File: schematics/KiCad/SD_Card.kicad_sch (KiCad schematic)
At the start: 13 parts, among them J6 Micro_SD_Card_Det_Hirose_DM3AT, U14 LP2950-3.3, U16 74HC4050

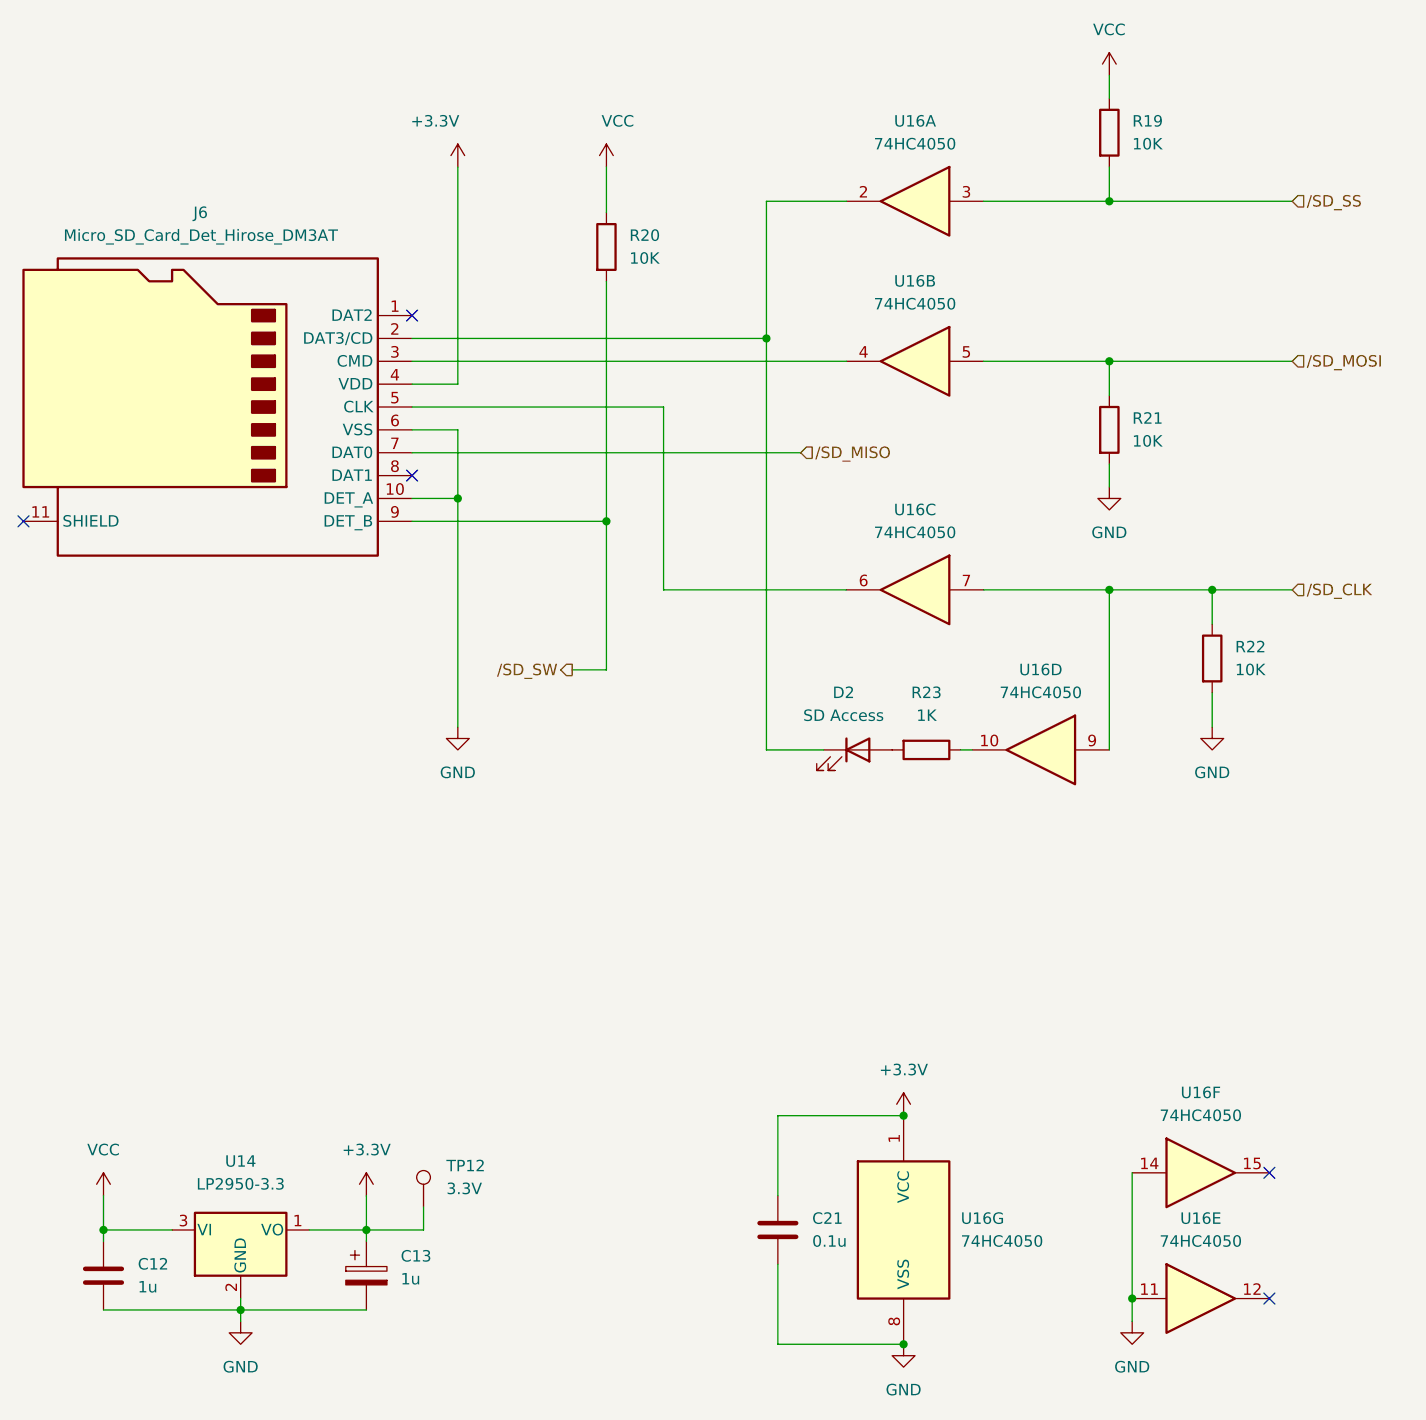
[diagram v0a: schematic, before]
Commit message: Update schematics
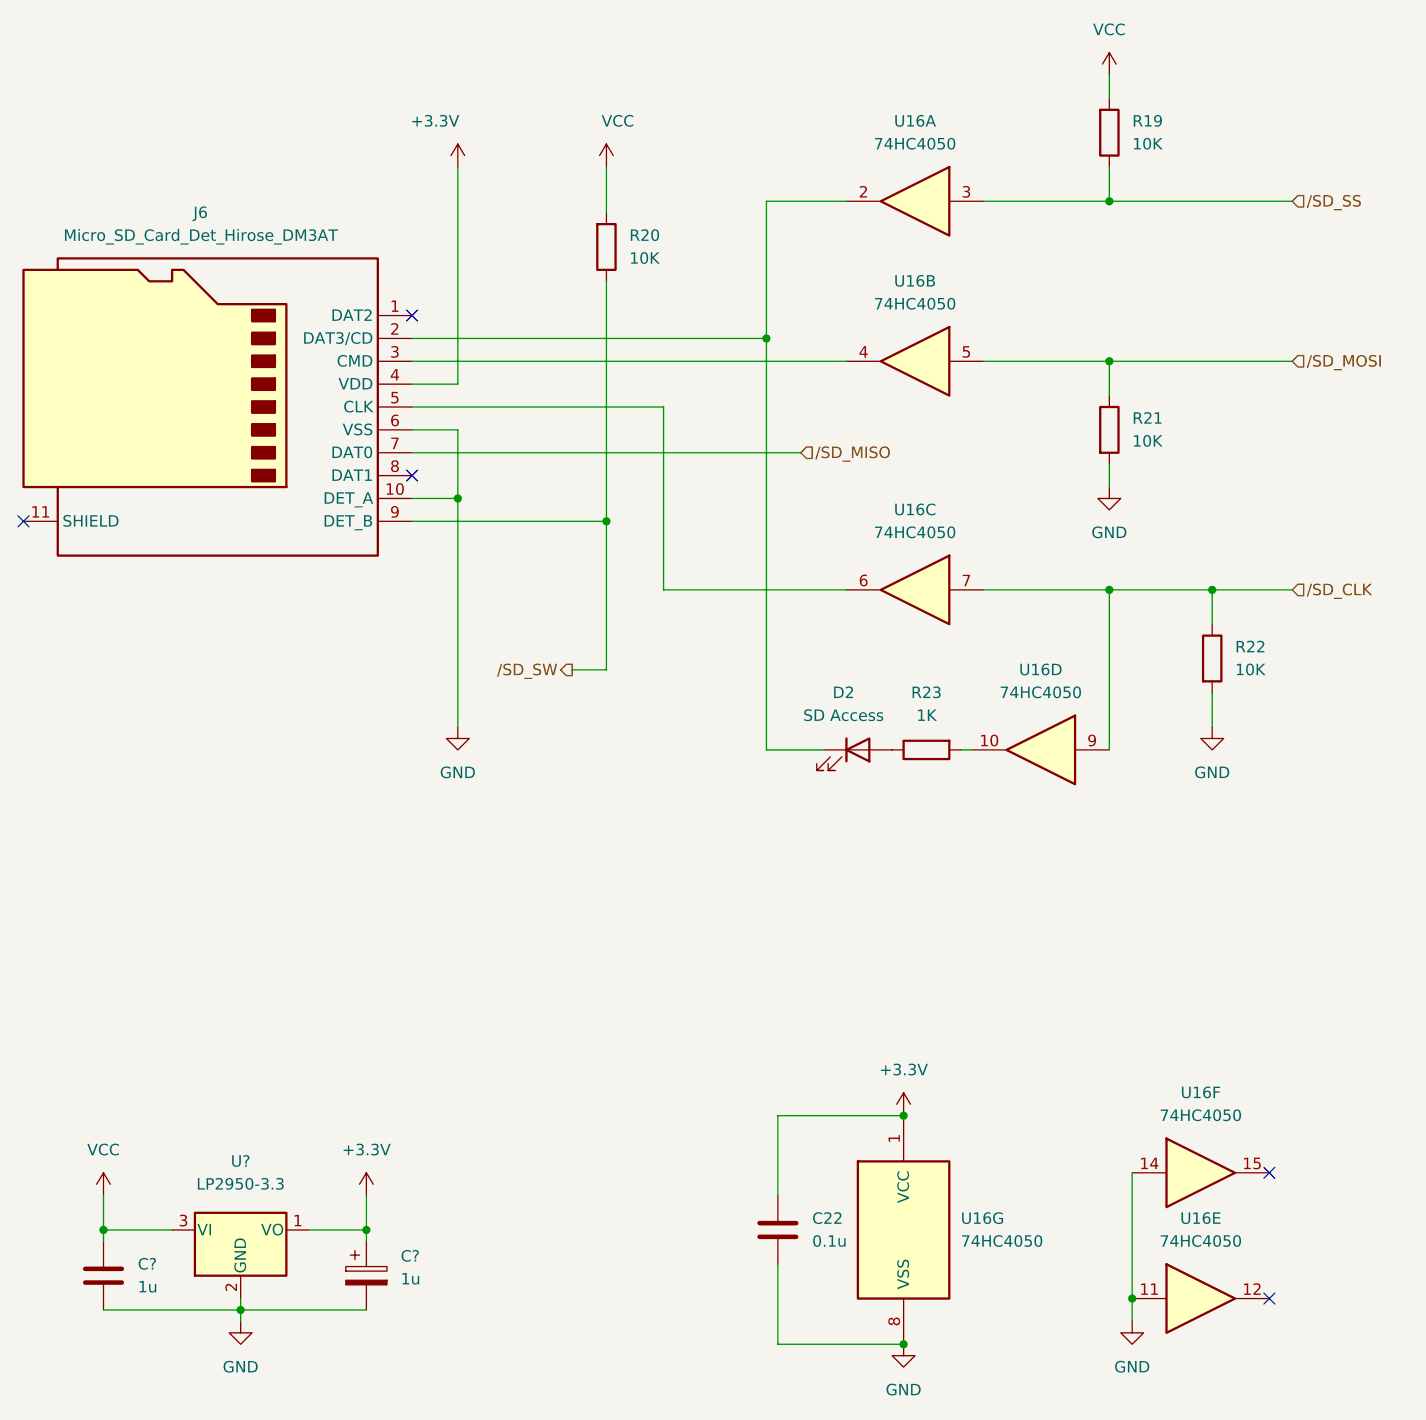
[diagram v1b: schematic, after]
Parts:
- removed TP12: 3.3V, TestPoint:TestPoint_Loop_D2.50mm_Drill1.0mm, symbol Connector:TestPoint
- C?: renamed from C12; footprint Capacitor_THT:CP_Radial_Tantal_D5.0mm_P2.50mm -> Capacitor_THT:C_Disc_D3.8mm_W2.6mm_P2.50mm
- C?: renamed from C13; footprint Capacitor_THT:CP_Radial_Tantal_D5.0mm_P2.50mm -> Capacitor_THT:CP_Radial_D5.0mm_P2.50mm
- renumbered C21 to C22, U14 to U?
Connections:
- net VCC: now also R19.2, R20.2; no longer R19.1, R20.1
- net /SD_SS: now also R19.1; no longer R19.2
- net /SD_SW: now also R20.1; no longer R20.2
- net at D2.2 (A): now also R23.1; no longer R23.2
- net at U16.10: now also R23.2; no longer R23.1
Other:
- moved on the sheet: R23

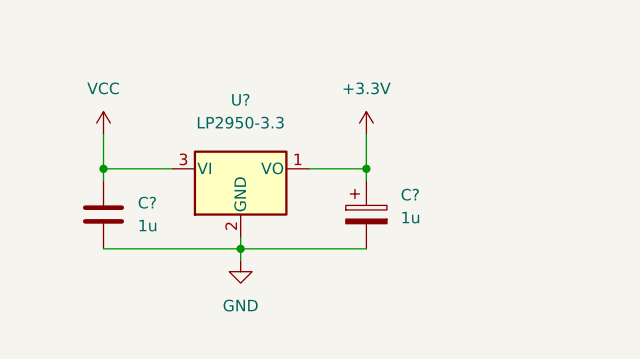
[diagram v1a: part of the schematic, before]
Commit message: Update for PCB design
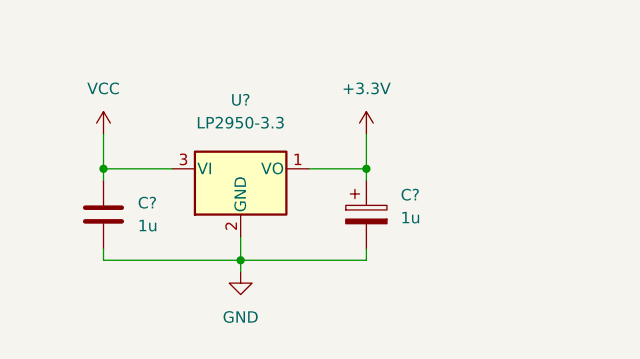
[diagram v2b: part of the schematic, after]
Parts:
- U?: footprint Package_TO_SOT_THT:TO-92_Inline -> Package_TO_SOT_THT:TO-92_Inline_Wide
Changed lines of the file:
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@@
     (company "By 46nori")
   )
-  (junction (at 49.53 167.64) (diameter 0) (color 0 0 0 0)
+  (junction (at 49.53 168.91) (diameter 0) (color 0 0 0 0)
   )
   (junction (at 107.95 59.69) (diameter 0) (color 0 0 0 0)
@@
     (stroke (width 0) (type default))
   )
+  (wire (pts (xy 63.5 168.91) (xy 63.5 167.64))
+    (stroke (width 0) (type default))
+  )
   (wire (pts (xy 109.22 162.56) (xy 109.22 171.45))
     (stroke (width 0) (type default))
@@
     (stroke (width 0) (type default))
   )
-  (wire (pts (xy 49.53 166.37) (xy 49.53 167.64))
-    (stroke (width 0) (type default))
-  )
-  (wire (pts (xy 49.53 167.64) (xy 63.5 167.64))
+  (wire (pts (xy 49.53 166.37) (xy 49.53 168.91))
+    (stroke (width 0) (type default))
+  )
+  (wire (pts (xy 49.53 168.91) (xy 63.5 168.91))
     (stroke (width 0) (type default))
   )
@@
     (stroke (width 0) (type default))
   )
+  (wire (pts (xy 34.29 168.91) (xy 34.29 167.64))
+    (stroke (width 0) (type default))
+  )
   (wire (pts (xy 129.54 105.41) (xy 130.81 105.41))
     (stroke (width 0) (type default))
@@
     (stroke (width 0) (type default))
   )
-  (wire (pts (xy 49.53 167.64) (xy 49.53 168.91))
+  (wire (pts (xy 49.53 168.91) (xy 49.53 170.18))
     (stroke (width 0) (type default))
   )
@@
     (stroke (width 0) (type default))
   )
-  (wire (pts (xy 34.29 167.64) (xy 49.53 167.64))
+  (wire (pts (xy 34.29 168.91) (xy 49.53 168.91))
     (stroke (width 0) (type default))
   )
@@
       (effects (font (size 1.27 1.27)))
     )
-    (property "Footprint" "Package_TO_SOT_THT:TO-92_Inline" (at 49.53 153.035 0)
+    (property "Footprint" "Package_TO_SOT_THT:TO-92_Inline_Wide" (at 49.53 153.035 0)
       (effects (font (size 1.27 1.27) italic) hide)
     )
@@
     )
   )
-  (symbol (lib_id "power:GND") (at 49.53 168.91 0) (unit 1)
-    (in_bom yes) (on_board yes) (dnp no) (fields_autoplaced)
-    (property "Reference" "#PWR?" (at 49.53 175.26 0)
-      (effects (font (size 1.27 1.27)) hide)
-    )
-    (property "Value" "GND" (at 49.53 173.99 0)
-      (effects (font (size 1.27 1.27)))
-    )
-    (property "Footprint" "" (at 49.53 168.91 0)
-      (effects (font (size 1.27 1.27)) hide)
-    )
-    (property "Datasheet" "" (at 49.53 168.91 0)
-      (effects (font (size 1.27 1.27)) hide)
-    )
+  (symbol (lib_id "power:GND") (at 49.53 170.18 0) (unit 1)
+    (in_bom yes) (on_board yes) (dnp no) (fields_autoplaced)
+    (property "Reference" "#PWR?" (at 49.53 176.53 0)
+      (effects (font (size 1.27 1.27)) hide)
+    )
+    (property "Value" "GND" (at 49.53 175.26 0)
+      (effects (font (size 1.27 1.27)))
+    )
+    (property "Footprint" "" (at 49.53 170.18 0)
+      (effects (font (size 1.27 1.27)) hide)
+    )
+    (property "Datasheet" "" (at 49.53 170.18 0)
+      (effects (font (size 1.27 1.27)) hide)
+    )
